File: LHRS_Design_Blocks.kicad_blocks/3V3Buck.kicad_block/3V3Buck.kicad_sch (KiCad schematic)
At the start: 28 parts, among them J1 SWD_Header_02x02, U2 STM32G491VET6_1, Y1 Crystal

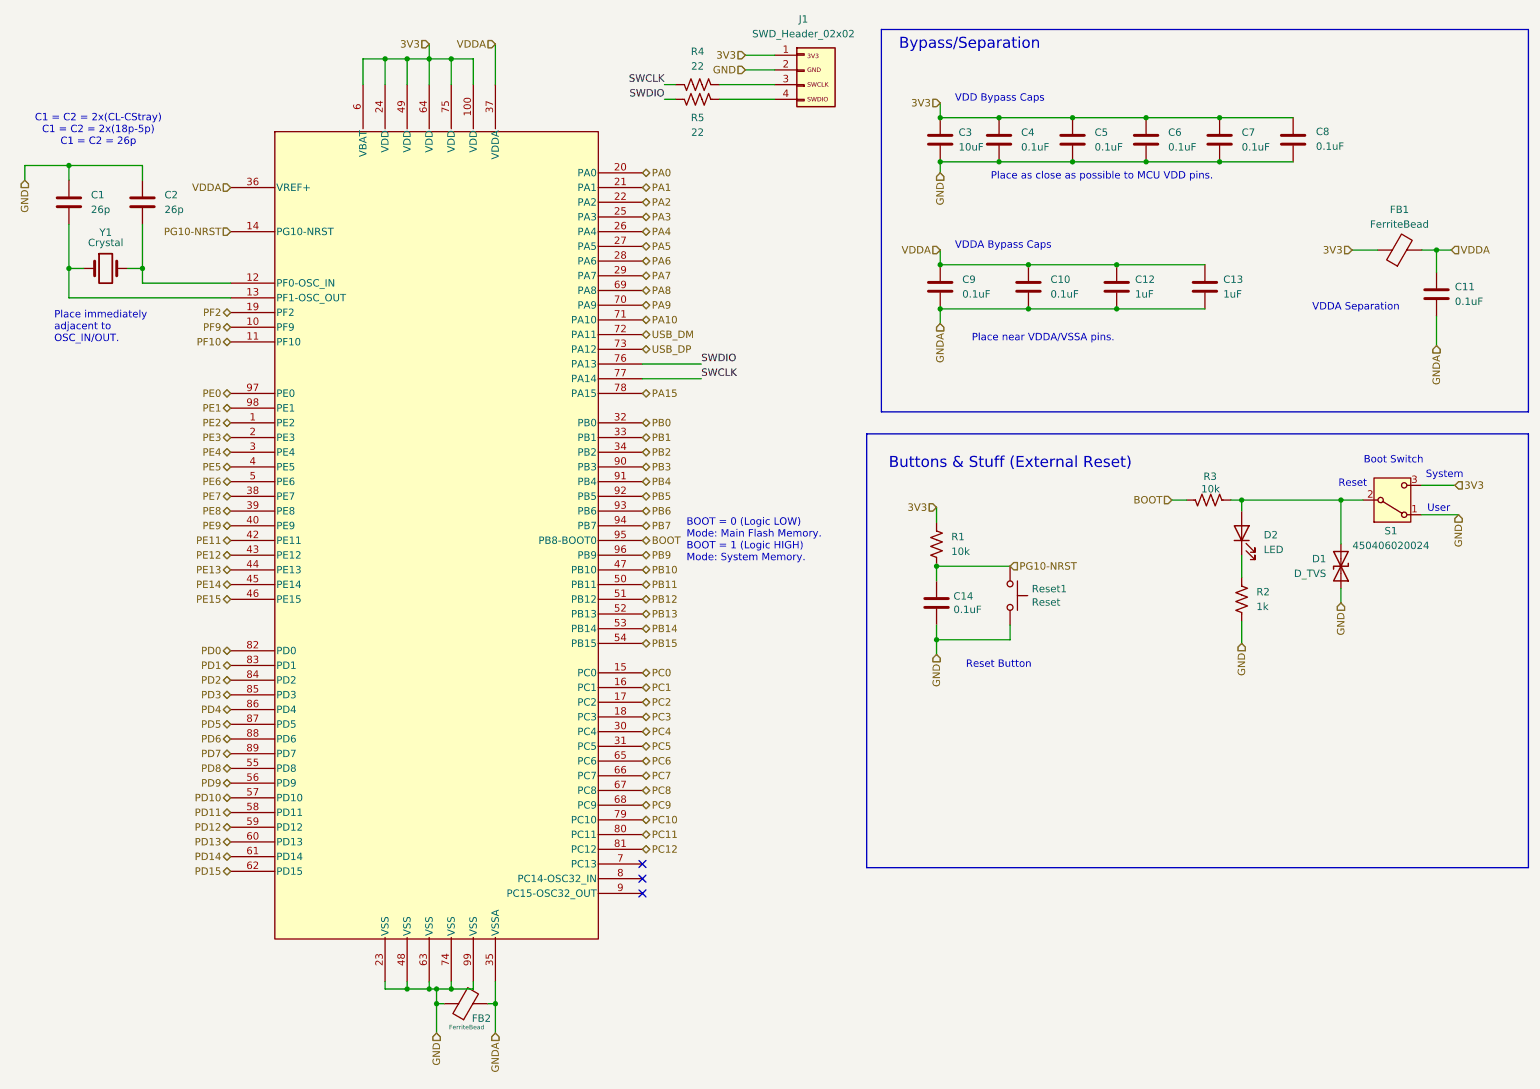
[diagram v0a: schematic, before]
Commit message: UTSVT to LHRS
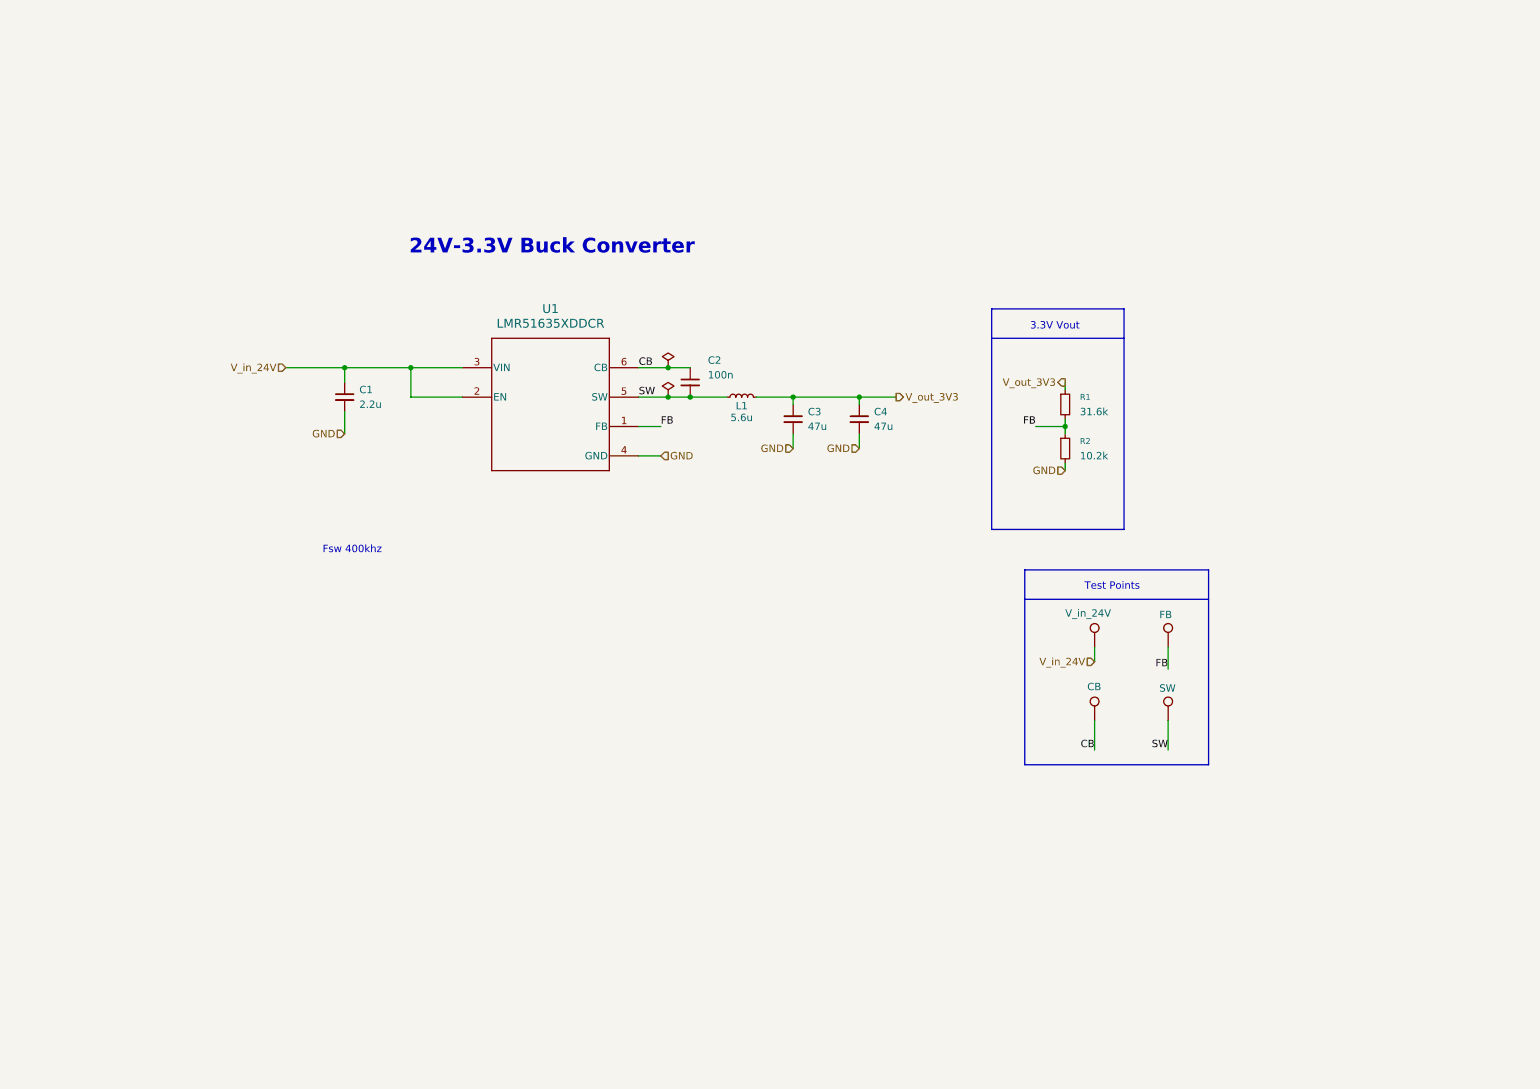
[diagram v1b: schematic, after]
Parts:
- removed C1, C2: 26p, Capacitor_SMD:C_0603_1608Metric_Pad1.08x0.95mm_HandSolder, symbol Device:C
- removed C10, C11, C14, C4, C5, C6, C7, C8, C9: 0.1uF, Capacitor_SMD:C_0603_1608Metric_Pad1.08x0.95mm_HandSolder, symbol Device:C
- removed C12, C13: 1uF, Capacitor_SMD:C_0603_1608Metric_Pad1.08x0.95mm_HandSolder, symbol Device:C
- removed C3: 10uF, Capacitor_SMD:C_0805_2012Metric, symbol Device:C
- removed D1: D_TVS, Diode_SMD:D_SOD-323, symbol Device:D_TVS
- removed D2: LED, LED_SMD:LED_0201_0603Metric, symbol Device:LED
- removed FB1, FB2: FerriteBead, Capacitor_SMD:C_0603_1608Metric_Pad1.08x0.95mm_HandSolder, symbol Device:FerriteBead
- removed J1: SWD_Header_02x02, UTSVT_Connectors:SWD_Conn, symbol 100PinMCU:SWD_Header_02x02
- removed R1, R3: 10k, Resistor_SMD:R_0603_1608Metric_Pad0.98x0.95mm_HandSolder, symbol Device:R_US
- removed R2: 1k, Resistor_SMD:R_0603_1608Metric_Pad0.98x0.95mm_HandSolder, symbol Device:R_US
- removed R4, R5: 22, Resistor_SMD:R_0603_1608Metric_Pad0.98x0.95mm_HandSolder, symbol Device:R_US
- removed Reset1: Reset, UTSVT_Special:TL3365AF180QG, symbol Switch:SW_Push
- removed S1: 450406020024, UTSVT_Special:BootSW, symbol Switch:SW_SPDT
- removed U2: STM32G491VET6_1, UTSVT_ICs:LQFP_491VET6_STM, symbol utsvt_ics:STM32G491VET6_1
- removed Y1: Crystal, UTSVT_Passives:Crystal_SMD_Abracon_ABM3-2Pin_5.0x3.2mm, symbol Device:Crystal
- added C1: 2.2u, Capacitor_SMD:C_0805_2012Metric_Pad1.18x1.45mm_HandSolder, symbol Device:C_Small
- added C2: 100n, Resistor_SMD:R_0201_0603Metric_Pad0.64x0.40mm_HandSolder, symbol Device:C_Small
- added C3, C4: 47u, Capacitor_SMD:C_1210_3225Metric_Pad1.33x2.70mm_HandSolder, symbol Device:C_Small
- added L1: 5.6u, Inductor_SMD:L_TDK_SLF6025, symbol Device:L_Small
- added R1: 31.6k, Resistor_SMD:R_0603_1608Metric, symbol Device:R_Small
- added R2: 10.2k, Resistor_SMD:R_0603_1608Metric, symbol Device:R_Small
- added TP?: FB, TestPoint:TestPoint_THTPad_D3.0mm_Drill1.5mm, symbol Connector:TestPoint
- added TP?: SW, TestPoint:TestPoint_THTPad_D3.0mm_Drill1.5mm, symbol Connector:TestPoint
- added TP?: CB, TestPoint:TestPoint_THTPad_D3.0mm_Drill1.5mm, symbol Connector:TestPoint
- added TP?: V_in_24V, TestPoint:TestPoint_THTPad_D3.0mm_Drill1.5mm, symbol Connector:TestPoint
- added U1: LMR51635XDDCR, LHRS_ICs:DDC0006A-MFG, symbol 2026-04-25_18-34-12:LMR51635XDDCR
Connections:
- net GND: now also C1.2, C3.2, C4.2, R2.2, U1.4 (GND)
- new net CB: C2.1, TP?.1, U1.6 (CB)
- new net FB: R1.2, R2.1, TP?.1, U1.1 (FB)
- new net SW: C2.2, L1.1, TP?.1, U1.5 (SW)
- new net V_in_24V: C1.1, TP?.1, U1.2 (EN), U1.3 (VIN)
- new net V_out_3V3: C3.1, C4.1, L1.2, R1.1
- no-connect marks 3 -> 0
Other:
- note added: "24V-3.3V Buck Converter"
- note added: "3.3V Vout"
- note added: "Fsw 400khz"
- note added: "Test Points"
- note removed: "BOOT = 0 (Logic LOW) Mode: Main Flash Memory. BOOT = 1 (Logic HIGH) Mode: System Memory."
- note removed: "Boot Switch"
- note removed: "Buttons & Stuff (External Reset)"
- note removed: "Bypass/Separation"
- note removed: "C1 = C2 = 2x(CL-CStray) C1 = C2 = 2x(18p-5p) C1 = C2 = 26p"
- note removed: "Place as close as possible to MCU VDD pins."
- note removed: "Place immediately adjacent to OSC_IN/OUT."
- note removed: "Place near VDDA/VSSA pins."
- note removed: "Reset"
- note removed: "Reset Button"
- note removed: "System"
- note removed: "User"
- note removed: "VDD Bypass Caps"
- note removed: "VDDA Bypass Caps"
- note removed: "VDDA Separation"
